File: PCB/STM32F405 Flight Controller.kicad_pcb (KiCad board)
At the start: 4 copper layers, 72.6 x 62.8 mm, 73 parts, among them J1 USB_C_Receptacle_USB2.0_16P, J2 XT60 (BATT), J3 ESC_1, J4 ESC_2, J5 ESC_3, J6 ESC_4, J7 SWD, SW1 SW_Push, SW2 SW_Push, U1 STM32F405RGTx, U2 MPU-6050, U3 BMP280, U4 AP7361C-33E, U5 LIS3MDL, U7 LMR33640DDDA, U8 W25Q128JVS, Y1 16MHz Crystal

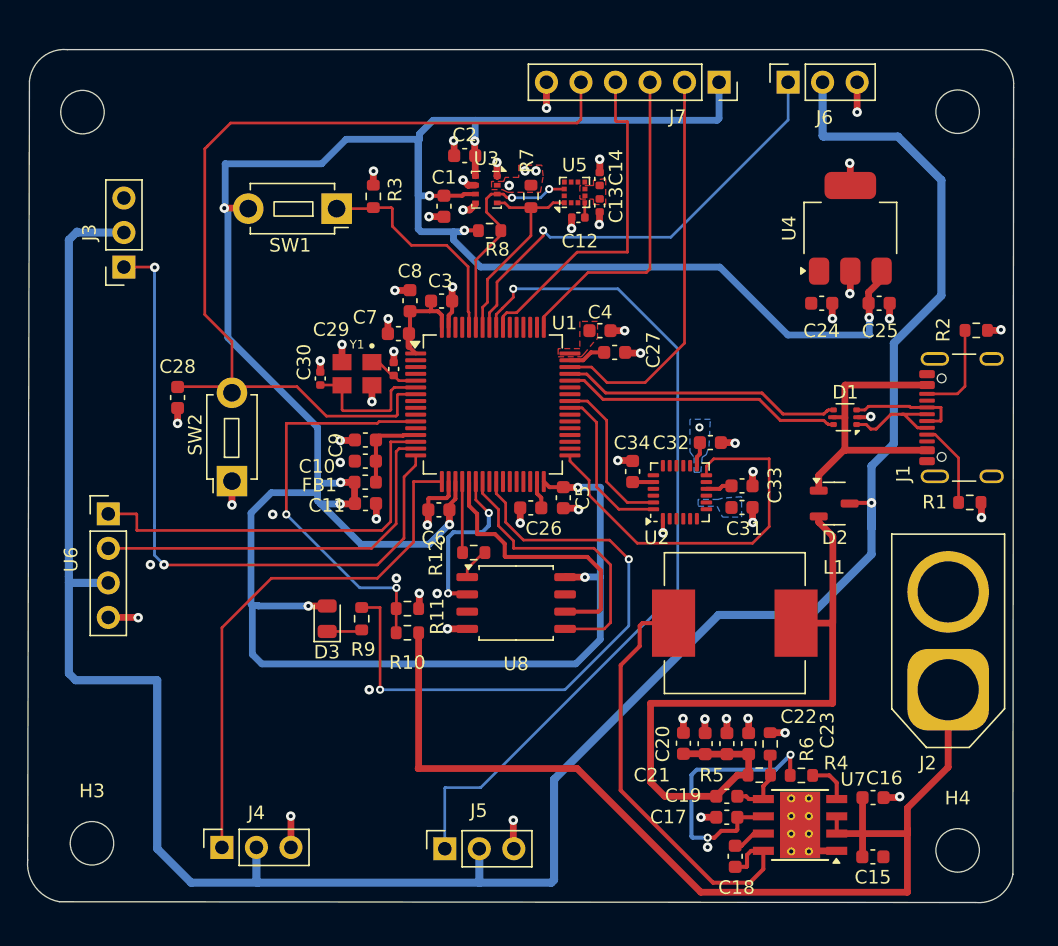
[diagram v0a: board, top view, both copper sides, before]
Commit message: Add files via upload
updated layout
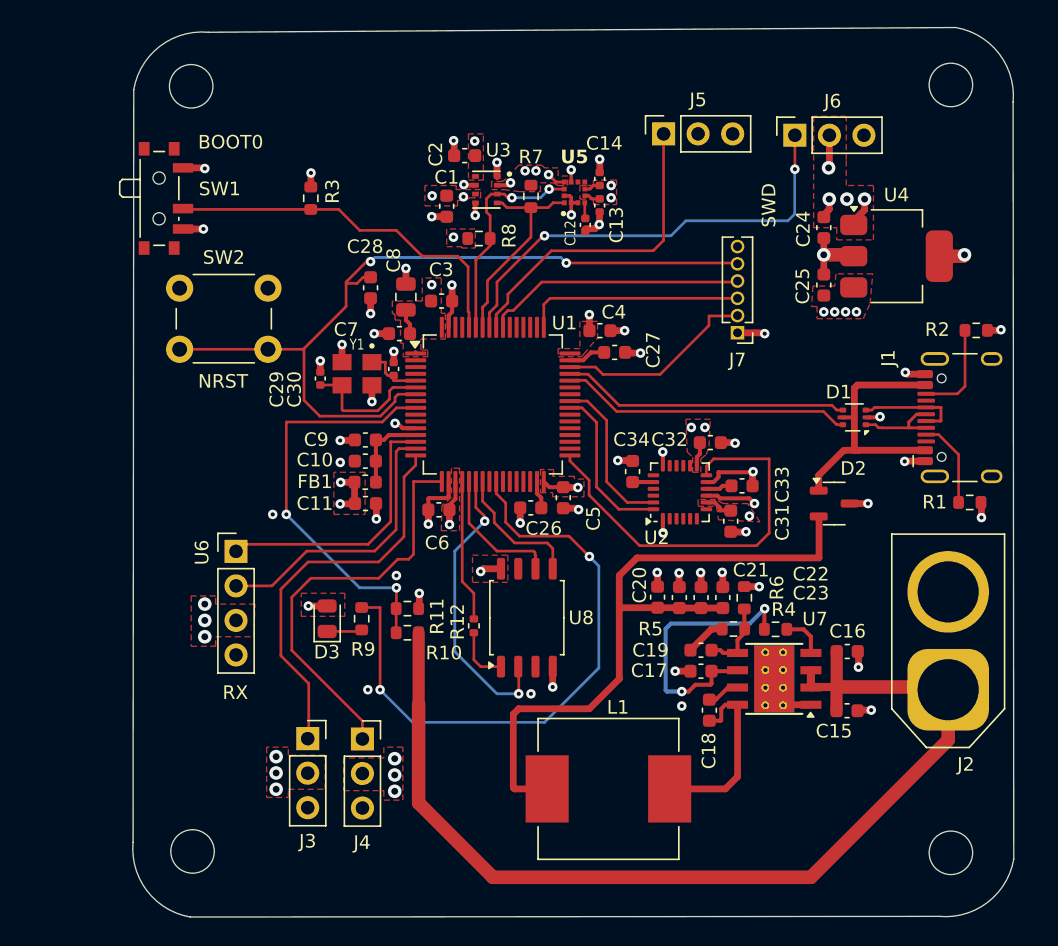
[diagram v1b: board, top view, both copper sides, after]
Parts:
- C29, C30: value 12pF -> 15pF
- C8: footprint Capacitor_SMD:C_0603_1608Metric -> Capacitor_SMD:C_0805_2012Metric
- J1: footprint Connector_USB:USB_C_Receptacle_GCT_USB4105-xx-A_16P_TopMnt_Horizontal -> Connector_USB:USB_C_Receptacle_HCTL_HC-TYPE-C-16P-01A
- J7: footprint Connector_PinSocket_2.54mm:PinSocket_1x06_P2.54mm_Vertical -> Connector_PinHeader_1.27mm:PinHeader_1x06_P1.27mm_Vertical
- R12: footprint Resistor_SMD:R_0603_1608Metric -> Resistor_SMD:R_0402_1005Metric
- SW1: value SW_Push -> SW_SPDT; footprint Button_Switch_THT:SW_PUSH_1P1T_6x3.5mm_H4.3_APEM_MJTP1243 -> Button_Switch_SMD:SW_SPDT_PCM12
- SW2: footprint Button_Switch_THT:SW_PUSH_1P1T_6x3.5mm_H4.3_APEM_MJTP1243 -> Button_Switch_THT:SW_PUSH_6mm_H4.3mm
- U3: footprint Package_LGA:Bosch_LGA-8_2x2.5mm_P0.65mm_ClockwisePinNumbering -> Custom Footprints:XDCR_BMP280
- U5: footprint Package_LGA:LGA-12_2x2mm_P0.5mm -> Custom Footprints:XDCR_LIS3MDL
- moved J5 55.0 mm to (162.3, 63.1)
- moved J3 37.2 mm to (136.1, 107.6), turned to 0 degrees
- moved J7 18.5 mm to (167.7, 77.7), turned to 180 degrees
- moved C28 16.3 mm to (140.7, 74.4)
- moved L1 15.3 mm to (158.2, 111.3), turned to 180 degrees
- moved SW2 14.7 mm to (126.7, 74.5), turned to 0 degrees
- moved J4 13.1 mm to (140.1, 107.6), turned to 0 degrees
- moved SW1 12.8 mm to (125.5, 67.8), turned to -90 degrees
- moved C15 10.9 mm to (175.8, 105.5)
- moved C16 10.9 mm to (175.8, 101.2)
- moved C17 10.9 mm to (165.0, 102.6)
- moved C18 10.9 mm to (165.6, 105.5)
- moved C20 10.9 mm to (161.8, 97.2)
- moved C21 10.9 mm to (163.4, 97.2)
- moved C22 10.9 mm to (165.0, 97.2)
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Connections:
- SW1 pad 1: BOOT0 -> +3.3V
- SW1 pad 2: +3.3V -> BOOT0
- U1 pad 11: BATT_SENSE -> unconnected-(U1-PC3-Pad11)
- U1 pad 9: unconnected-(U1-PC1-Pad9) -> BATT_SENSE
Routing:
- net +3.3V: track 230.3 -> 190.3 mm, vias 15 -> 27
- net ESC_3: track 62.7 -> 23.7 mm, vias 1 -> 0
- net ESC_1: track 49.4 -> 28.9 mm, vias 2 -> 0
- net Net-(U7-SW): track 33.4 -> 13.7 mm
- net +5V: track 179.7 -> 163.0 mm, vias 1 -> 14
- net SWDIO: track 29.3 -> 14.8 mm
- net MOSI: track 21.3 -> 9.96 mm
- net SCK: track 21.2 -> 10.0 mm
- net BOOT0: track 16.8 -> 27.2 mm
- net UART1_TX: track 29.9 -> 19.7 mm
- net NRST: track 70.4 -> 60.5 mm, vias 0 -> 2
- net ESC_2: track 39.4 -> 30.3 mm
- net MISO: track 12.6 -> 21.7 mm
- net GND: track 69.8 -> 78.2 mm, vias 58 -> 57
- net UART1_RX: track 28.8 -> 20.8 mm
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- added copper zone on F.Cu, net +5V
- removed copper zone on B.Cu, net +3.3V
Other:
- board size 72.6 x 62.8 mm -> 64.8 x 65.5 mm
- board text added: "BOOT0"
- board text added: "NRST"
- board text added: "RX"
- board text added: "SWD"

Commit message: Add files via upload
updated layout
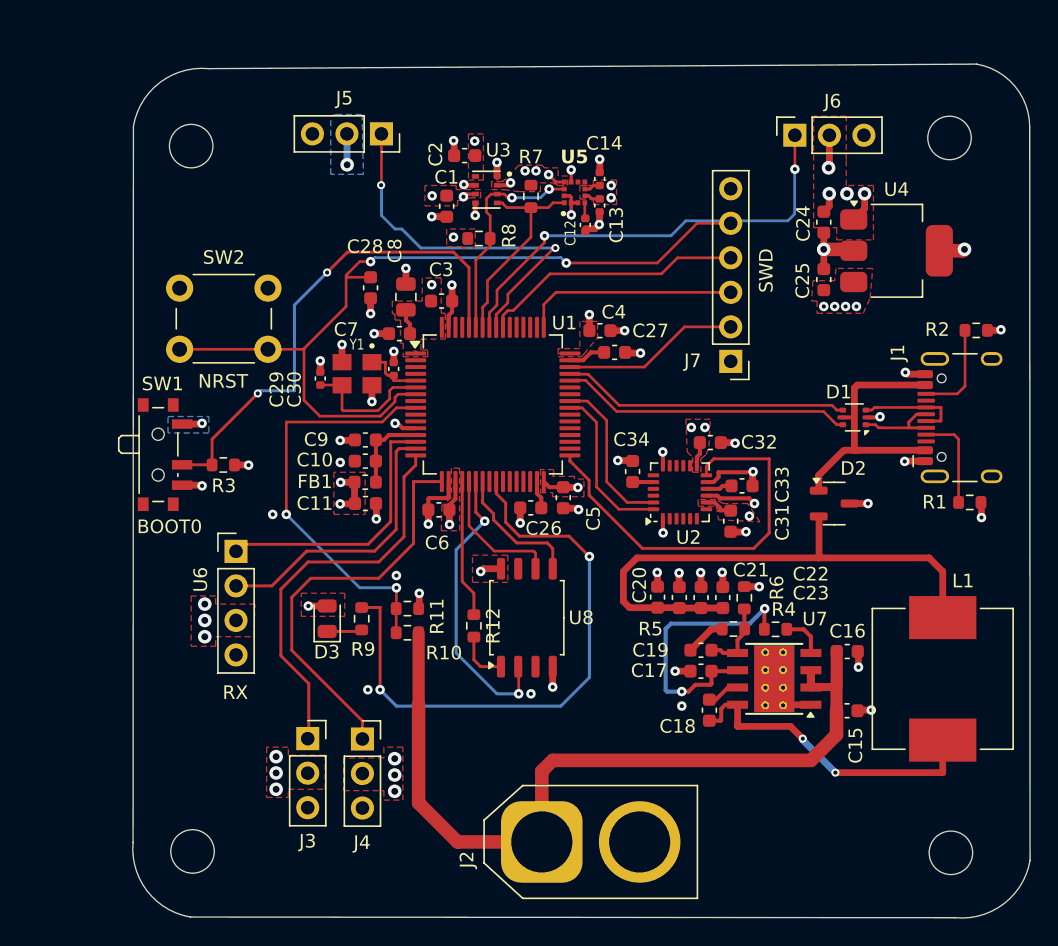
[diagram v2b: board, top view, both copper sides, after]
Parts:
- J7: footprint Connector_PinHeader_1.27mm:PinHeader_1x06_P1.27mm_Vertical -> Connector_PinHeader_2.54mm:PinHeader_1x06_P2.54mm_Vertical
- R12: footprint Resistor_SMD:R_0402_1005Metric -> Resistor_SMD:R_0603_1608Metric
- moved J2 31.9 mm to (153.3, 115.2), turned to 0 degrees
- moved L1 25.9 mm to (182.8, 103.2), turned to 90 degrees
- moved J5 20.8 mm to (141.5, 63.1), turned to -90 degrees
- moved R3 20.7 mm to (129.9, 87.5), turned to 180 degrees
- moved SW1 18.9 mm to (125.4, 86.7)
- moved H1 4.40 mm to (127.5, 64.0)
- moved H2 3.90 mm to (183.3, 63.4)
- moved J7 2.16 mm to (167.2, 79.8)
- moved C24 0.40 mm to (174.1, 69.6)
- moved C25 0.40 mm to (174.1, 73.8)
- moved U4 0.40 mm to (179.4, 71.7)
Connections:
- net +5V_BATT renamed Net-(D2-A1)
- net +5V_VBUS renamed Net-(D1-VP)
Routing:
- net +BATT: track 79.2 -> 60.3 mm
- net +3.3V: track 190.3 -> 171.6 mm, vias 27 -> 26
- net +5V: track 163.0 -> 177.4 mm, vias 14 -> 15
- net BOOT0: track 27.2 -> 37.3 mm, vias 0 -> 2
- net Net-(U7-SW): track 13.7 -> 23.6 mm, vias 0 -> 2
- net Net-(D2-A1): track 53.8 -> 44.0 mm
- net ESC_3: track 23.7 -> 27.5 mm, vias 0 -> 2
- net SWDIO: track 14.8 -> 13.1 mm
- net Net-(U1-PC5): track 45.1 -> 43.6 mm
- net NRST: track 60.5 -> 61.3 mm
- net Net-(J1-CC1): track 6.52 -> 7.18 mm
- added copper zone on B.Cu, net +3.3V
- added copper zone on B.Cu, net +5V
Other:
- board size 64.8 x 65.5 mm -> 66 x 62.8 mm
